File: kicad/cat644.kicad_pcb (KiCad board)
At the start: 2 copper layers, 101.6 x 76.2 mm, 42 parts, among them P2 PWR, P3 ISP, P4 SER, P5 SD, P6 PS2, P7 AUD, P8 VGA, U1 ATMEGA644-P, U2 74LS573, U3 628128, U4 74LS244, U5 7805, U6 SPX2920U-3.3, U7 MAX232, U8 74LS244, X1 OSC 20MHz

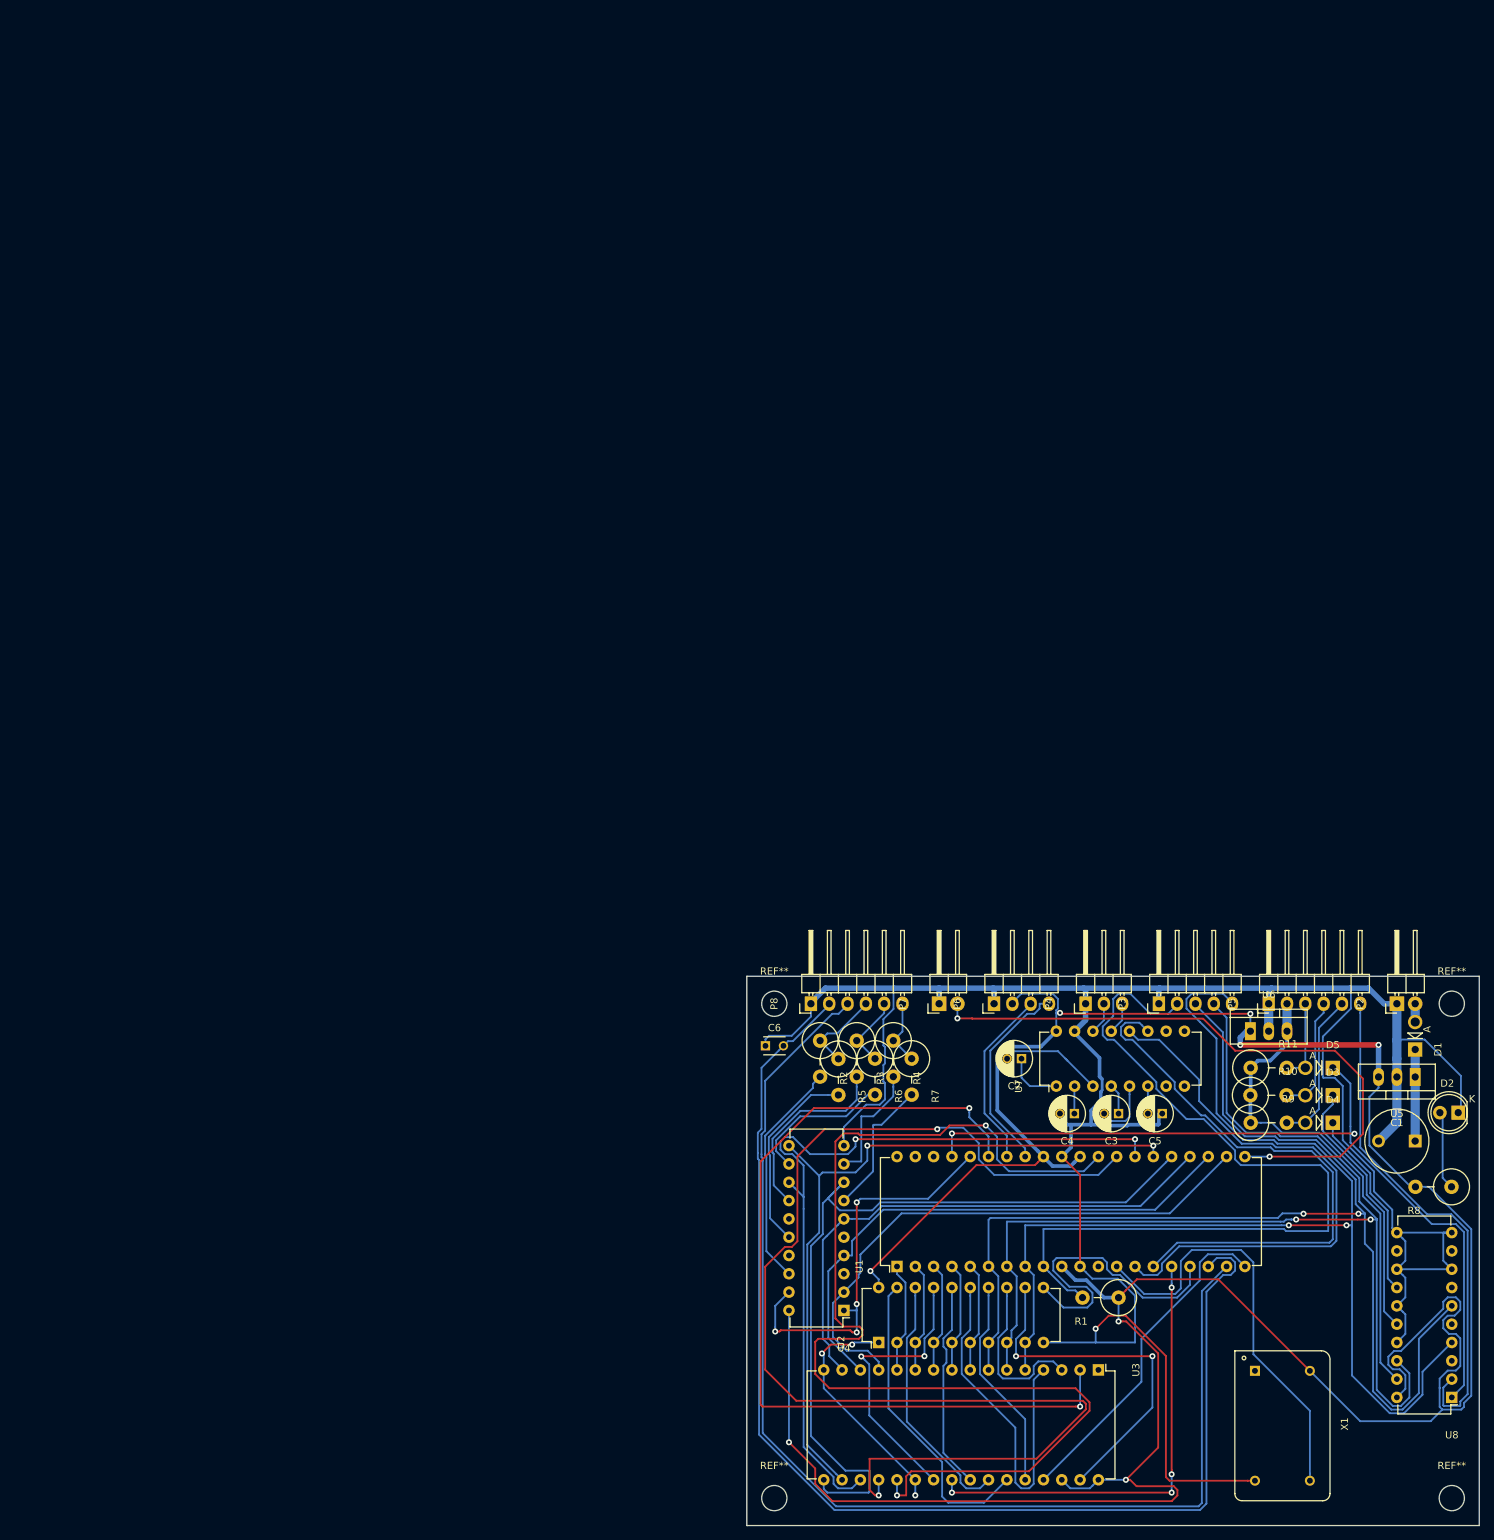
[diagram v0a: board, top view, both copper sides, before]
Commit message: updated pcb
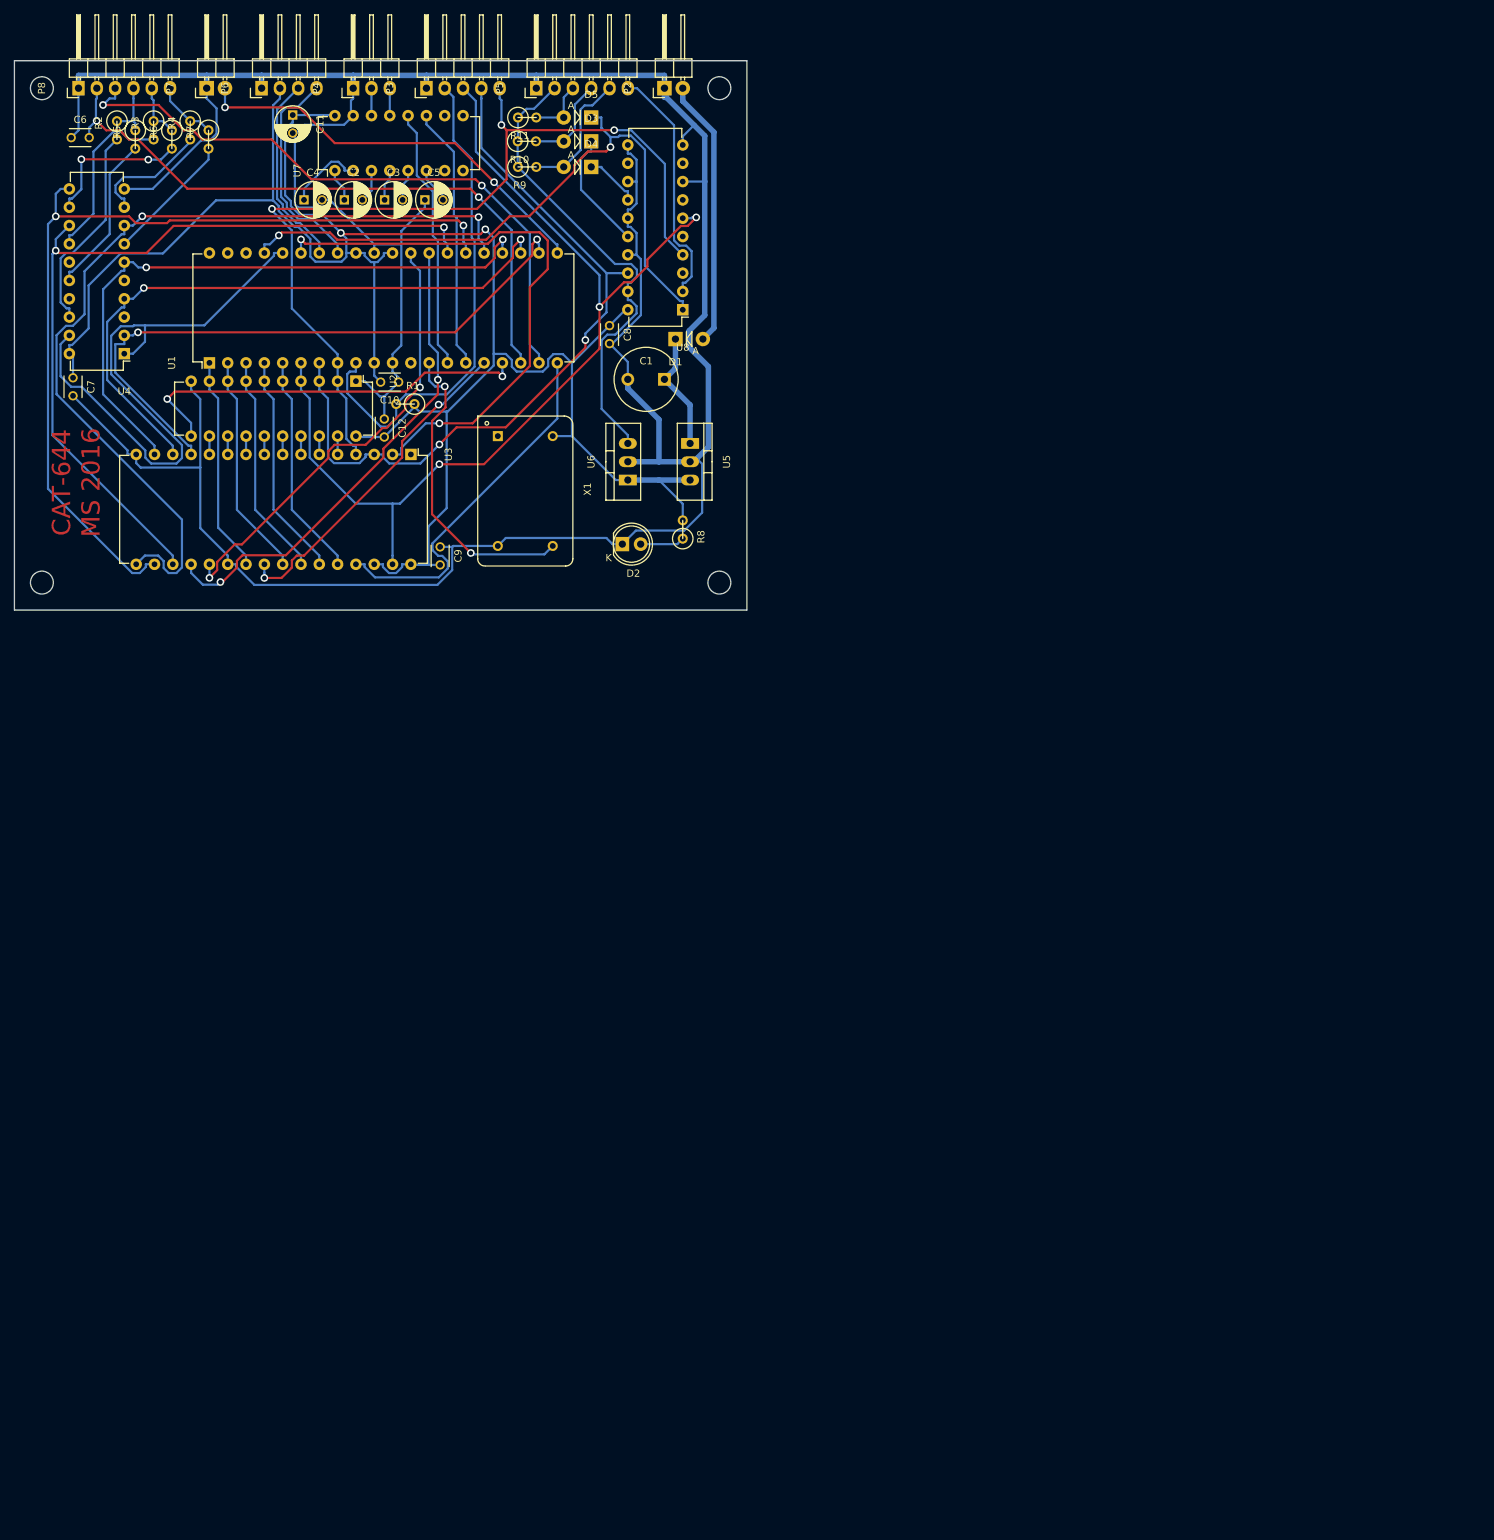
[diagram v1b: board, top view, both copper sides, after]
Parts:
- removed REF** (x4): MountingHole_3.5mm, Mounting_Holes:MountingHole_3.5mm
- added C10: 0.1uF, Capacitors_ThroughHole:C_Disc_D3_P2.5, F.Cu at (53.3, -31.6)
- added C11: 10uF, Capacitors_ThroughHole:C_Radial_D5_L11_P2.5, F.Cu at (38.6, -68.7)
- added C12: 0.1uF, Capacitors_ThroughHole:C_Disc_D3_P2.5, F.Cu at (51.3, -26.5)
- added C7: 0.1uF, Capacitors_ThroughHole:C_Disc_D3_P2.5, F.Cu at (8.13, -32.2)
- added C8: 0.1uF, Capacitors_ThroughHole:C_Disc_D3_P2.5, F.Cu at (82.5, -39.5)
- added C9: 0.1uF, Capacitors_ThroughHole:C_Disc_D3_P2.5, F.Cu at (59.1, -8.76)
- added mh1: MountingHole_3.5mm, Mounting_Holes:MountingHole_3.5mm, F.Cu at (3.81, -3.81)
- added mh2: MountingHole_3.5mm, Mounting_Holes:MountingHole_3.5mm, F.Cu at (97.8, -3.81)
- added mh3: MountingHole_3.5mm, Mounting_Holes:MountingHole_3.5mm, F.Cu at (97.8, -72.4)
- added mh4: MountingHole_3.5mm, Mounting_Holes:MountingHole_3.5mm, F.Cu at (3.81, -72.4)
- C2, C3, C4, C5: footprint Capacitors_ThroughHole:C_Radial_D5_L11_P2 -> Capacitors_ThroughHole:C_Radial_D5_L11_P2.5
- R1, R10, R11, R2, R3, R4, R5, R6, R7, R8, R9: footprint Resistors_ThroughHole:Resistor_Vertical_RM5mm -> Discret:R1
- moved U8 184.8 mm to (92.7, -41.7)
- moved R9 167.8 mm to (71.1, -61.5)
- moved D4 167.8 mm to (80.0, -61.5)
- moved R10 167.6 mm to (71.1, -65.0)
- moved D3 167.6 mm to (80.0, -65.0)
- moved D5 167.2 mm to (80.0, -68.3)
- moved R11 167.2 mm to (71.1, -68.3)
- moved X1 166.9 mm to (70.9, -16.5)
- moved U4 166.1 mm to (15.2, -35.6)
- moved C4 165.8 mm to (40.2, -56.9), turned to 0 degrees
- moved C5 162.9 mm to (56.9, -56.9), turned to 0 degrees
- moved P2 162.6 mm to (90.2, -72.4)
- moved P3 162.6 mm to (57.1, -72.4)
- moved P4 162.6 mm to (47.0, -72.4)
- moved P5 162.6 mm to (72.4, -72.4)
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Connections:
- U1 pad 12: Net-(U1-Pad12) -> (no net)
- U1 pad 38: Net-(U1-Pad38) -> (no net)
- U1 pad 39: Net-(U1-Pad39) -> (no net)
- U1 pad 40: Net-(U1-Pad40) -> (no net)
- U2 pad 2: Net-(U1-Pad1) -> /serial/SCLK
- U2 pad 3: Net-(U1-Pad2) -> /serial/MISO
- U2 pad 4: Net-(U1-Pad3) -> /serial/MOSI
- U2 pad 5: Net-(U1-Pad4) -> Net-(U1-Pad5)
- U2 pad 6: Net-(U1-Pad5) -> Net-(U1-Pad4)
- U2 pad 7: /serial/MOSI -> Net-(U1-Pad3)
- U2 pad 8: /serial/MISO -> Net-(U1-Pad2)
- U2 pad 9: /serial/SCLK -> Net-(U1-Pad1)
- U3 pad 10: Net-(U1-Pad3) -> Net-(U2-Pad14)
- U3 pad 11: Net-(U1-Pad2) -> Net-(U2-Pad13)
- U3 pad 12: Net-(U1-Pad1) -> Net-(U2-Pad12)
- U3 pad 23: Net-(U2-Pad17) -> Net-(U1-Pad1)
- U3 pad 25: Net-(U2-Pad16) -> Net-(U1-Pad2)
- U3 pad 26: Net-(U2-Pad18) -> Net-(U1-Pad3)
- U3 pad 27: Net-(U2-Pad19) -> Net-(U1-Pad4)
- U3 pad 28: Net-(U2-Pad14) -> Net-(U1-Pad5)
- U3 pad 3: Net-(U2-Pad13) -> /serial/MISO
- U3 pad 31: Net-(U2-Pad12) -> /serial/MOSI
- U3 pad 4: Net-(U2-Pad15) -> /serial/SCLK
- U3 pad 5: /serial/SCLK -> Net-(U2-Pad19)
- U3 pad 6: /serial/MISO -> Net-(U2-Pad18)
- U3 pad 7: /serial/MOSI -> Net-(U2-Pad17)
- U3 pad 8: Net-(U1-Pad5) -> Net-(U2-Pad16)
- U3 pad 9: Net-(U1-Pad4) -> Net-(U2-Pad15)
- U4 pad 15: Net-(U4-Pad15) -> (no net)
- U4 pad 17: Net-(U4-Pad17) -> (no net)
- U4 pad 3: Net-(U4-Pad3) -> (no net)
- U4 pad 5: Net-(U4-Pad5) -> (no net)
- U7 pad 10: Net-(U7-Pad10) -> (no net)
- U7 pad 7: Net-(U7-Pad7) -> (no net)
- U7 pad 8: Net-(U7-Pad8) -> (no net)
- U7 pad 9: Net-(U7-Pad9) -> (no net)
- U8 pad 12: Net-(U8-Pad12) -> (no net)
- U8 pad 3: Net-(U8-Pad3) -> (no net)
- U8 pad 5: Net-(U8-Pad5) -> (no net)
- U8 pad 7: Net-(U8-Pad7) -> (no net)
- U8 pad 9: Net-(U8-Pad9) -> (no net)
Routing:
- net VCC: track 422.6 -> 293.8 mm, vias 8 -> 2
- net Net-(U1-Pad28): track 171.2 -> 68.4 mm
- net Net-(U1-Pad29): track 160.1 -> 63.1 mm
- net /av/VSYNC: track 171.4 -> 90.2 mm, vias 0 -> 2
- net /av/HSYNC: track 164.6 -> 88.5 mm, vias 0 -> 2
- net /serial/MISO: track 153.5 -> 105.1 mm
- net Net-(U2-Pad12): track 50.3 -> 2.54 mm, vias 2 -> 0
- net Net-(U2-Pad15): track 50.1 -> 2.54 mm
- net /serial/RESET: track 117.2 -> 69.7 mm
- net GND: track 417.5 -> 464.8 mm, vias 4 -> 0
- net /serial/TX1_IN: track 79.2 -> 36.6 mm
- net /serial/RX1_OUT: track 79.1 -> 36.6 mm
- net Net-(U1-Pad35): track 123.1 -> 80.6 mm
- net Net-(U2-Pad19): track 43.2 -> 2.54 mm
- net /serial/SCLK: track 162.9 -> 123.9 mm, vias 2 -> 3
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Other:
- net class Default: trace_width 0.254 -> 0.3048; via_dia 0.8382 -> 1.0668; via_drill 0.4 -> 0.8128
- net class power removed
- board text added: "CAT-644 MS 2016"
